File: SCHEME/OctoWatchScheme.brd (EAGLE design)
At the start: 35 x 34 mm, 24 parts, among them IC1 TP4056, IC2 DS1302, J1 0475900001, Y2 32.768kHz

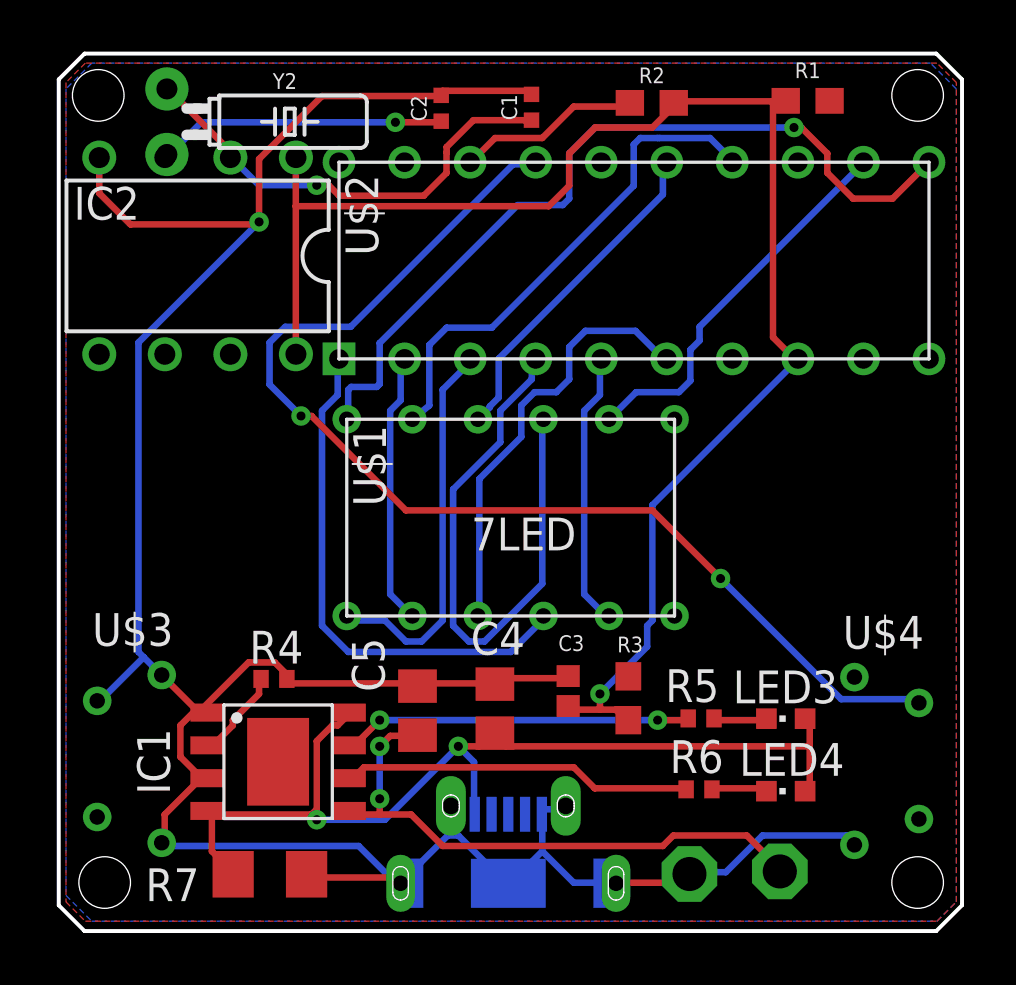
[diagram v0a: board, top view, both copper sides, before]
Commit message: Adding new package
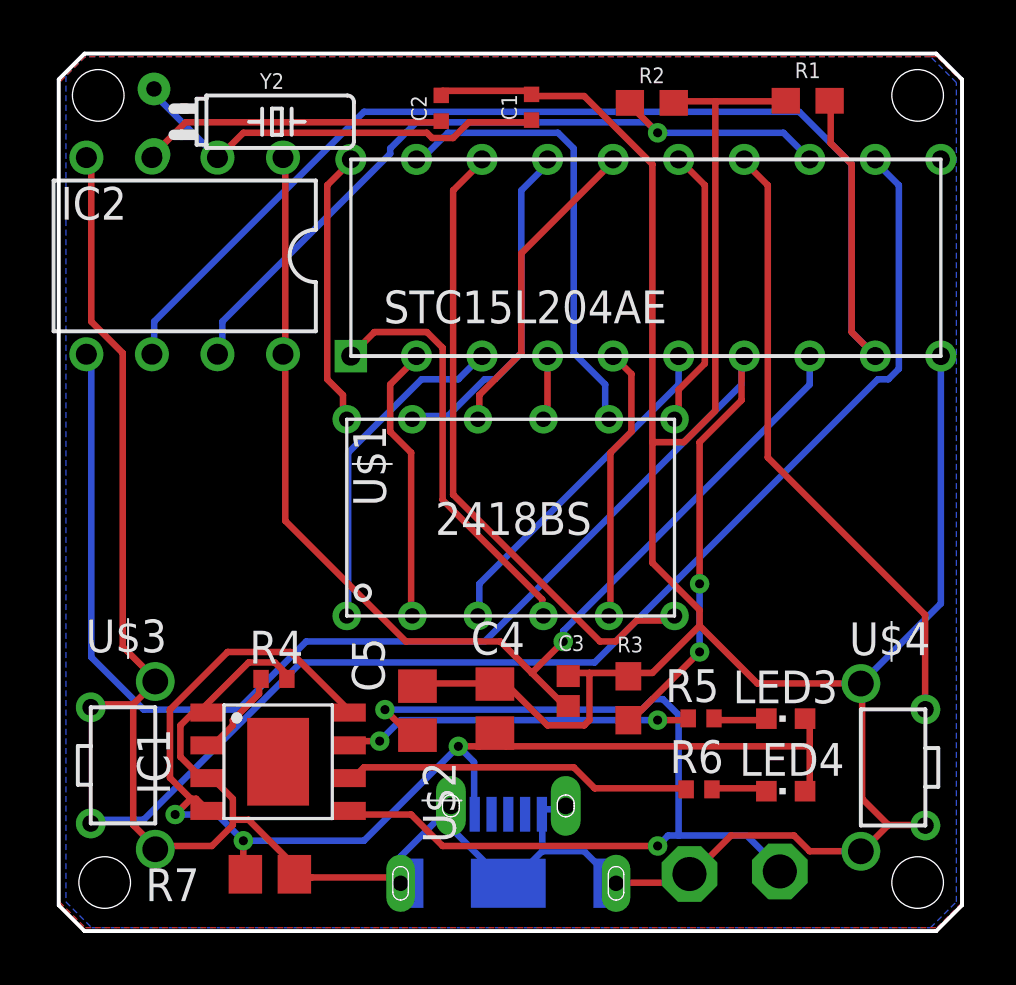
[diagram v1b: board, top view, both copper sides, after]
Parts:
- R7: device rcl:R1206 -> rcl:R0805
- U$2: device OctoWatch:STC15F204AE -> OctoWatch:STC15F204AE2
- moved U$2 22.9 mm to (50.7, 58.1)
- moved IC2 0.50 mm to (34.1, 49.3)
- moved Y2 0.50 mm to (32.9, 54.5)
- moved U$3 0.35 mm to (21.5, 31.8)
- moved U$4 0.35 mm to (71.8, 27.2)
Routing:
- net GND: track 109.3 -> 175.1 mm, vias 1 -> 0
- net N$14: track 0.00 -> 60.3 mm, vias 0 -> 2
- net N$17: track 0.00 -> 51.0 mm
- net N$20: track 0.00 -> 47.1 mm
- net N$6: track 0.00 -> 24.8 mm
- net N$23: track 7.14 -> 29.9 mm, vias 0 -> 1
- net N$7: track 32.0 -> 10.8 mm, vias 1 -> 0
- net N$19: track 45.1 -> 24.2 mm, vias 2 -> 0
- net N$10: track 22.7 -> 2.53 mm
- net N$18: track 22.3 -> 36.3 mm
- net BATT+: track 58.3 -> 44.9 mm
- net N$32: track 38.4 -> 50.2 mm, vias 2 -> 3
- net N$12: track 0.00 -> 11.0 mm
- net N$8: track 19.6 -> 13.2 mm
- net N$3: track 20.2 -> 16.2 mm
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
